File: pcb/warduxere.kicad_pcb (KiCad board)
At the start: 2 copper layers, 35 parts, among them IC2 ATMEGA328P-A, K1 CONN_3, P1 UART-USB, U1 MCP1700 3.3V

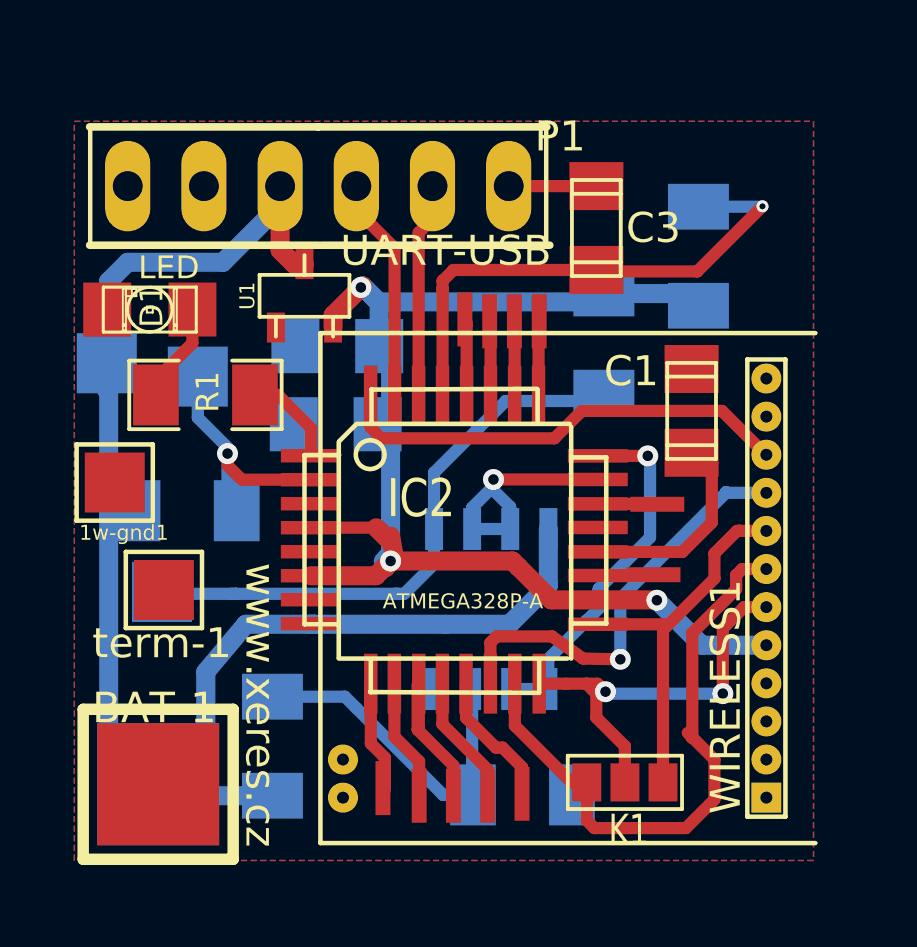
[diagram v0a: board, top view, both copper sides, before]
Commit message: DPS version2
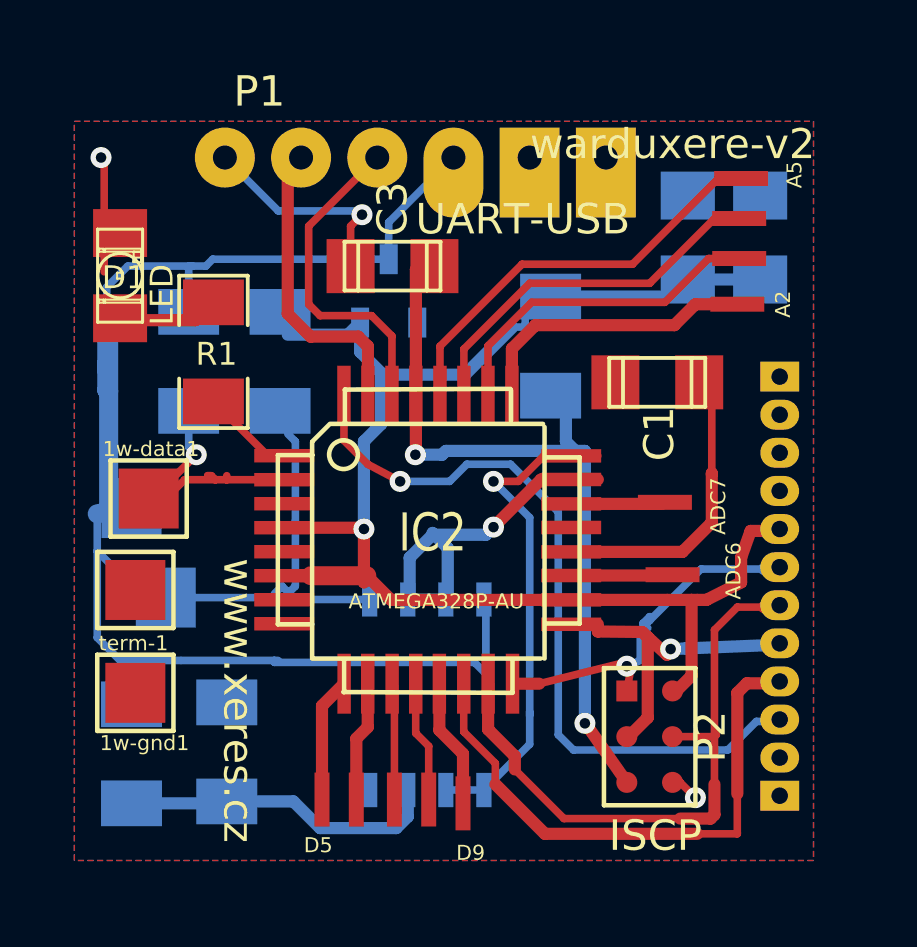
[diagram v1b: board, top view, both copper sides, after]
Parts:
- removed BAT+1, BAT-1: CONN_1, 1PIN_SMD
- removed K1: CONN_3, GS3
- added P2: ISCP, pin_array_3x2X-ISCP, F.Cu at (88.5, 69.8)
- 1w-data1: moved to F.Cu
- IC2: value ATMEGA328P-A -> ATMEGA328P-AU
- OP1: value MCP6042 -> MCP6042-I/SN; footprint SO8E -> SO8N
- P1: footprint PINHEAD1-6x -> PINHEAD1-6x+
- R2, R4: value 10k -> 10K
- R3: value 4k7 -> 4K7
- R5: value 10k -> 1M
- R6: value 10K -> 1M
- U1: value MCP1700 3.3V -> MCP1700T-3302E/TT; moved to B.Cu
- WIRELESS1: moved to B.Cu
- moved C4 15.5 mm to (92.2, 53.1), turned to 270 degrees
- moved C2 12.2 mm to (89.8, 53.1), turned to 270 degrees
- moved R4 10.8 mm to (76.2, 57.3)
- moved A5 10.3 mm to (91.6, 51.2), turned to 90 degrees
- moved R6 9.96 mm to (74.4, 70.3), turned to 90 degrees
- moved A4 9.00 mm to (91.5, 52.5), turned to 90 degrees
- moved A3 7.78 mm to (91.5, 53.8), turned to 90 degrees
- moved 1w-gnd1 7.04 mm to (71.4, 68.3)
- moved C3 6.91 mm to (79.9, 54.1), turned to 180 degrees
- moved A2 6.63 mm to (91.4, 55.4), turned to 90 degrees
- moved R2 5.77 mm to (85.2, 56.8), turned to 270 degrees
- moved R3 4.98 mm to (73.2, 57.3), turned to 270 degrees
- moved 1w-vcc1 4.90 mm to (71.2, 62.2)
- moved R5 4.71 mm to (71.2, 70.4), turned to 270 degrees
- moved 1w-data1 4.38 mm to (71.8, 61.8)
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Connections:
- net VCC renamed +3.3V
- IC2 pad 30: N-0000030 (its old number) -> N-0000035
- IC2 pad 31: N-0000029 (its old number) -> N-0000023
- P1 pad 2: N-0000030 (its old number) -> N-0000023
- P1 pad 3: N-0000029 (its old number) -> N-0000035
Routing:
- net N-0000025: track 2.42 -> 14.0 mm
- net N-000002: track 15.4 -> 26.7 mm, vias 0 -> 1
- net N-0000035: track 0.00 -> 11.0 mm
- net N-0000023: track 0.00 -> 10.2 mm
- net N-0000026: track 2.43 -> 12.5 mm
- net N-0000030: track 2.42 -> 11.2 mm
- net N-000009: track 17.7 -> 25.4 mm, vias 1 -> 2
- net N-0000029 (its old number): track 7.51 -> 0.00 mm
- net N-0000031: track 2.42 -> 9.69 mm
- net N-0000030 (its old number): track 7.18 -> 0.00 mm
- net GND: track 0.00 -> 6.34 mm, vias 0 -> 2
- net +3.3V: track 44.3 -> 49.4 mm, vias 3 -> 1
- net N-000006: track 18.2 -> 13.4 mm
- net N-0000013: track 14.5 -> 19.2 mm, vias 1 -> 0
- net N-0000027: track 2.92 -> 7.23 mm, vias 0 -> 1
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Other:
- board text added: "warduxere-v2"
